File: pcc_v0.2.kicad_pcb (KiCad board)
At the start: 2 copper layers, 170.3 x 151.7 mm, 69 parts, among them J2 Conn_01x04_Socket, J3 Conn_01x02_Socket, J4 Conn_02x14_Counter_Clockwise, J6 Conn_01x04_Socket, J7 Conn_01x04_Socket, J8 Conn_01x02_Socket, K3 PCN-112D3MHZ_000, K4 Relay_SPDT, U10 LM2904B, U2 4N35, U3 4N35, U5 DMN63D8L-7, U8 SN65HVD230, U9 LM1117T-5.0

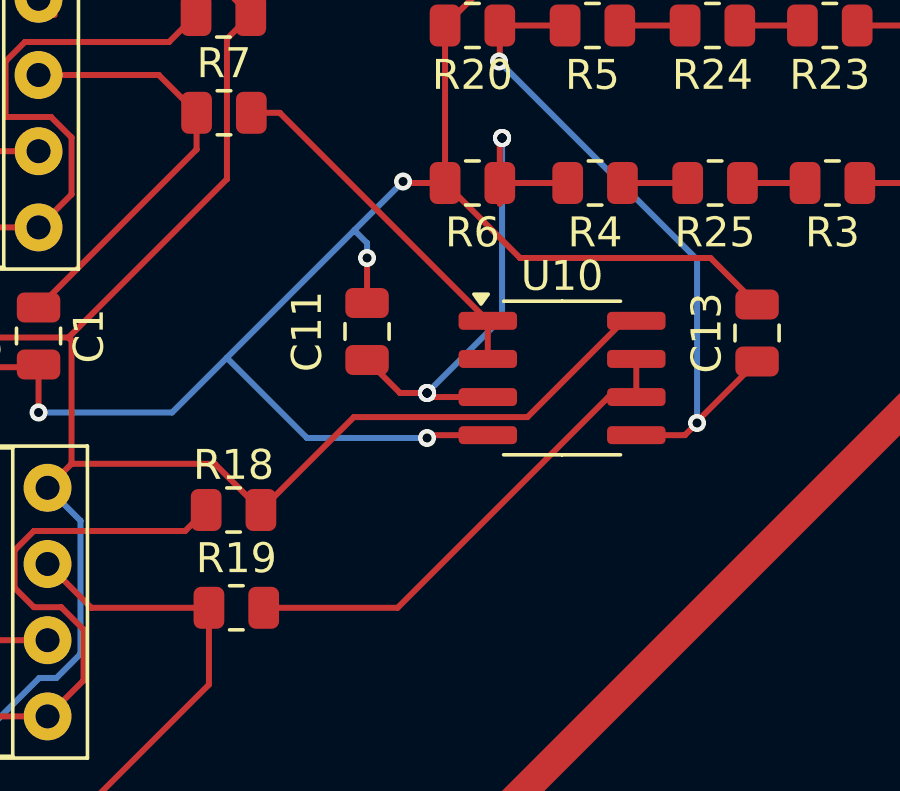
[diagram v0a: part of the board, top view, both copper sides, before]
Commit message: Add files via upload
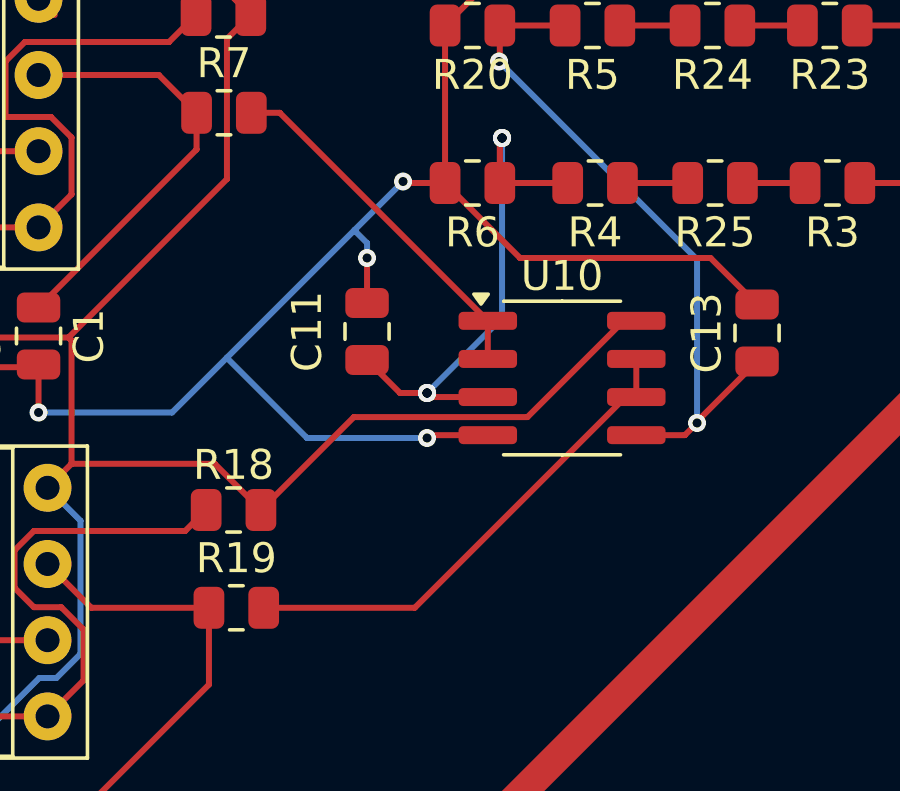
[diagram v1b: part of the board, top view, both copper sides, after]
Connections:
- J6 pad 3: TS- -> TS+
- J6 pad 4: TS+ -> TS-
- R21 pad 1: TS- -> TS+
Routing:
- net TS-: track 162.3 -> 134.6 mm
- net TS+: track 134.6 -> 162.3 mm
- net Net-(U10A-+): track 18.6 -> 17.9 mm
